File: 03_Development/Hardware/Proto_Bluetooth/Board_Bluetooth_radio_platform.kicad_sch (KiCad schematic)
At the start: 48 parts, among them J1 Conn_01x02, J10 Conn_01x03, J11 HMI_rotaryEncoder_1, J12 HMI_rotaryEncoder_1, J13 Conn_01x08_epaper, J19 Conn_01x02_rn52_usb, J2 Conn_01x08, J3 BT_RN52_connector_left, J4 Conn_01x02, J5 BT_RN52_connector_right, J6 FM_interface, J7 BT_debug_connector, J8 BT_extension_connector, J9 SYS_debug_connector, SW1 SW_Push, U1 LM317_TO-220

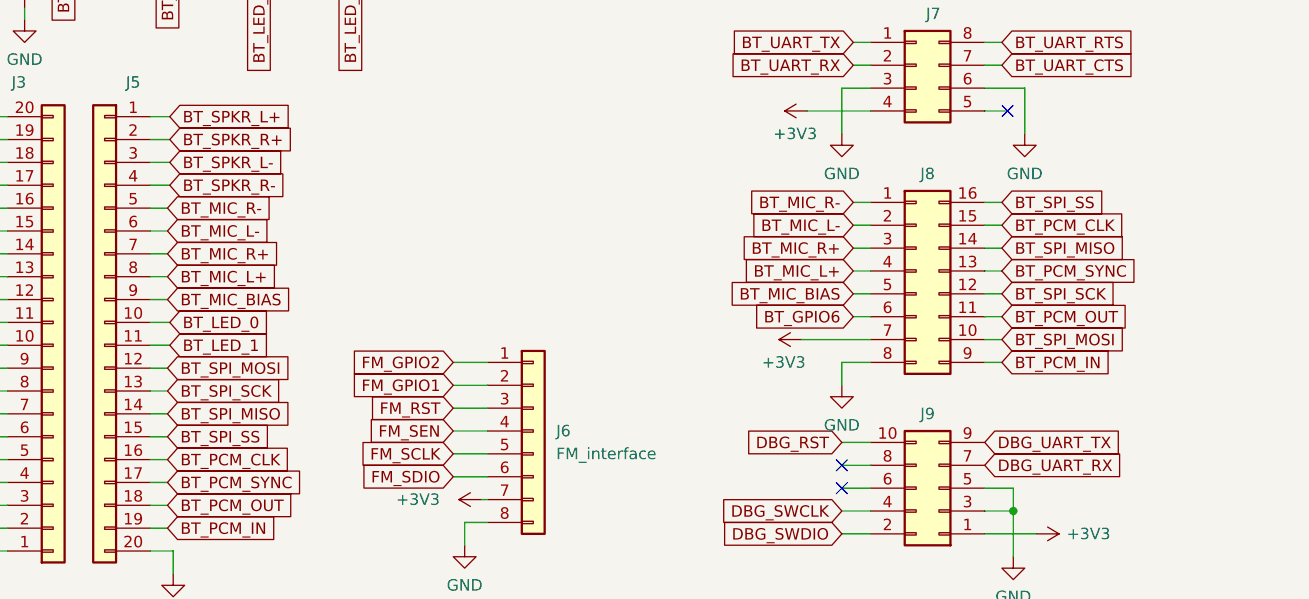
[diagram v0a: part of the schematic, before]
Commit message: [HDW_49] FIX place of elements for new version
Remove micro i/o from RN52 as they won't be used
Move power supply down on PCB
Move class D amplifier
Add hole for push buttons mounting
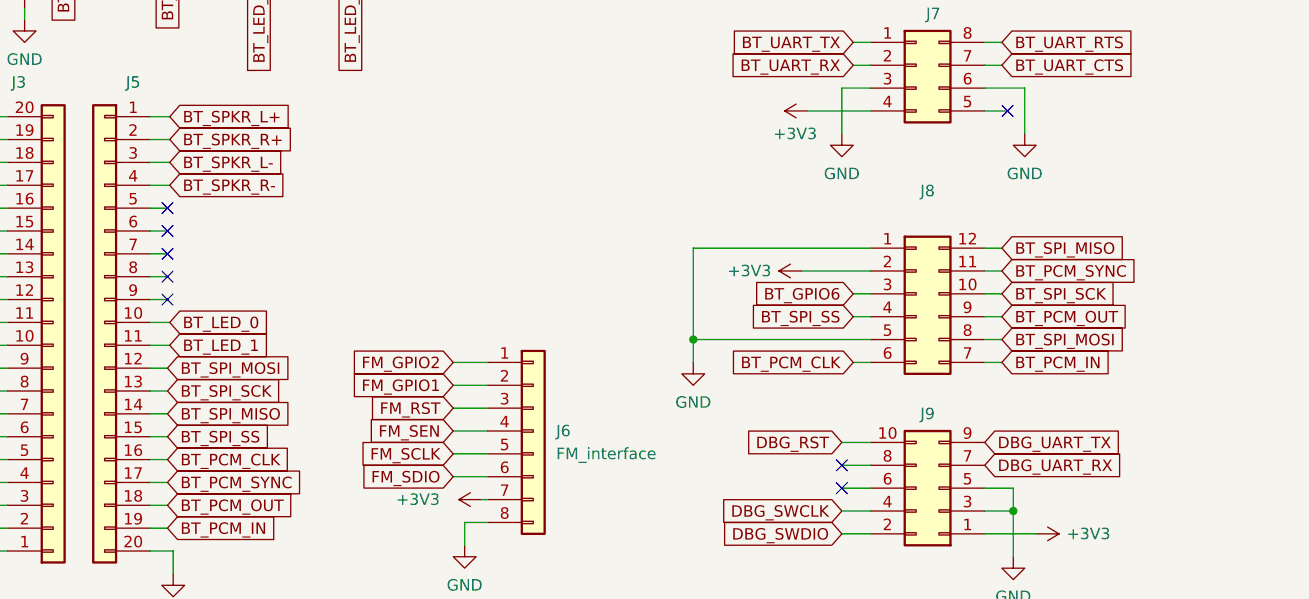
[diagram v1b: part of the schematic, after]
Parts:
- removed J8: BT_extension_connector, Connector_PinSocket_2.54mm:PinSocket_2x08_P2.54mm_Vertical, symbol Connector_Generic:Conn_02x08_Counter_Clockwise
- added J8: Conn_02x06_Counter_Clockwise, Connector_PinSocket_2.54mm:PinSocket_2x06_P2.54mm_Vertical, symbol Connector_Generic:Conn_02x06_Counter_Clockwise
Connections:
- net +3V3: now also J8.2 (Pin_2)
- net BT_GPIO6: now also J8.3 (Pin_3)
- net BT_PCM_CLK: now also J8.6 (Pin_6)
- net BT_PCM_IN: now also J8.7 (Pin_7)
- net BT_PCM_OUT: now also J8.9 (Pin_9)
- net BT_PCM_SYNC: now also J8.11 (Pin_11)
- net BT_SPI_MISO: now also J8.12 (Pin_12)
- net BT_SPI_MOSI: now also J8.8 (Pin_8)
- net BT_SPI_SCK: now also J8.10 (Pin_10)
- net BT_SPI_SS: now also J8.4 (Pin_4)
- net GND: now also J8.1 (Pin_1), J8.5 (Pin_5)
- net BT_MIC_BIAS: no longer names the net of J5.9 (Pin_9)
- net BT_MIC_L+: no longer names the net of J5.8 (Pin_8)
- net BT_MIC_L-: no longer names the net of J5.6 (Pin_6)
- net BT_MIC_R+: no longer names the net of J5.7 (Pin_7)
- net BT_MIC_R-: no longer names the net of J5.5 (Pin_5)
- no-connect marks 10 -> 15

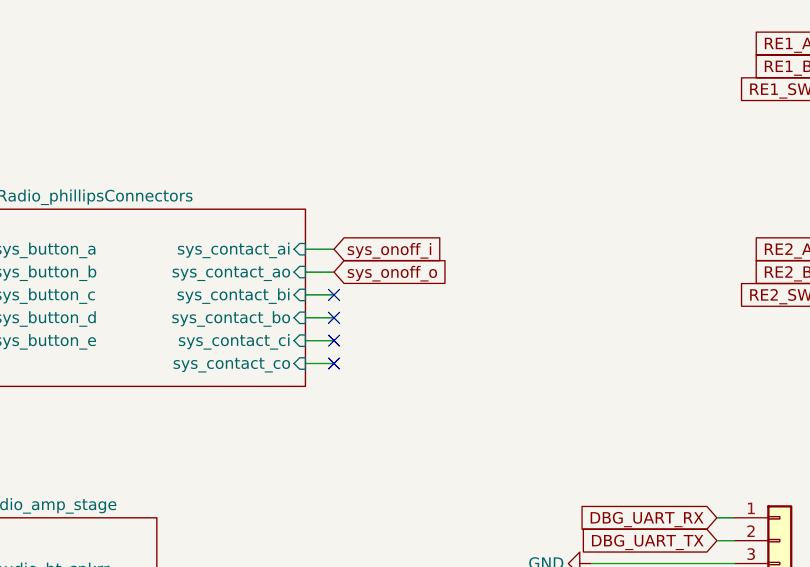
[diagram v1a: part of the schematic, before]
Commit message: [HDW_51] FIX push button connector
Push button connector for power supply was not a holding
one and had to be changed to a holding one
PCB updated
Add of GND to some of the headers
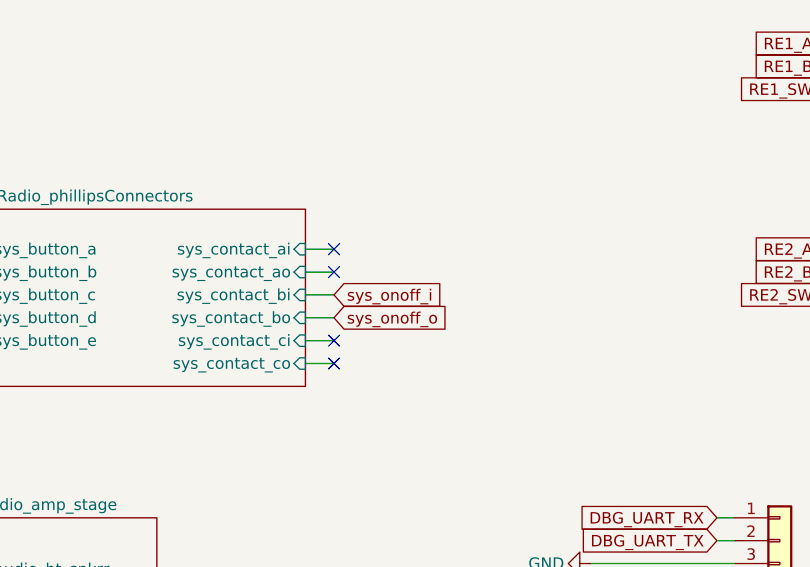
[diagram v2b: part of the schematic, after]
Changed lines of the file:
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@@
   )
   (no_connect (at 137.16 78.105))
-  (no_connect (at 180.975 78.105))
+  (no_connect (at 180.975 73.025))
   (no_connect (at 153.035 142.24))
   (no_connect (at 59.69 158.115))
-  (no_connect (at 180.975 75.565))
+  (no_connect (at 180.975 70.485))
   (no_connect (at 59.69 163.195))
   (no_connect (at 180.975 83.185))
@@
     )
   )
-  (global_label "sys_onoff_i" (shape input) (at 180.975 70.485 0) (fields_autoplaced)
+  (global_label "sys_onoff_i" (shape input) (at 180.975 75.565 0) (fields_autoplaced)
     (effects (font (size 1.27 1.27)) (justify left))
-    (property "Intersheet References" "${INTERSHEET_REFS}" (id 0) (at 193.8505 70.4056 0)
+    (property "Intersheet References" "${INTERSHEET_REFS}" (id 0) (at 193.8505 75.4856 0)
       (effects (font (size 1.27 1.27)) (justify left) hide)
     )
@@
     )
   )
-  (global_label "sys_onoff_o" (shape input) (at 180.975 73.025 0) (fields_autoplaced)
+  (global_label "sys_onoff_o" (shape input) (at 180.975 78.105 0) (fields_autoplaced)
     (effects (font (size 1.27 1.27)) (justify left))
-    (property "Intersheet References" "${INTERSHEET_REFS}" (id 0) (at 194.3948 72.9456 0)
+    (property "Intersheet References" "${INTERSHEET_REFS}" (id 0) (at 194.3948 78.0256 0)
       (effects (font (size 1.27 1.27)) (justify left) hide)
     )
@@
       (reference "#PWR0166") (unit 1) (value "+3V3") (footprint "")
     )
+    (path "/f502a33a-d5e4-4b91-95a6-ac6a3abcb73b/4cee3fe2-7a49-4ea3-8dc4-0f7703510c06"
+      (reference "#PWR?") (unit 1) (value "GND") (footprint "")
+    )
+    (path "/f502a33a-d5e4-4b91-95a6-ac6a3abcb73b/557cc4f9-b02c-474b-91ea-cad4e36f9b5a"
+      (reference "#PWR?") (unit 1) (value "GND") (footprint "")
+    )
+    (path "/f502a33a-d5e4-4b91-95a6-ac6a3abcb73b/f4336b9f-7927-4d47-9509-dd3fd3c54804"
+      (reference "#PWR?") (unit 1) (value "GND") (footprint "")
+    )
     (path "/5a833556-9b2d-4a89-ade5-f769671d3e3c"
